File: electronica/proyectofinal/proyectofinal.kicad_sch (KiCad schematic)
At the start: 16 parts, among them J1 cnn, J2 conector alimentacion esp, J3 dht22, J4 Guva-s12s, J5 convertidor_TTL, J6 MICS-6814, K1 SRD-05VDC-SL-C, K2 SRD-05VDC-SL-C, U1 LM7833_TO220, U3 LM7805_TO220, U4 ESP32_LORA_V2.0

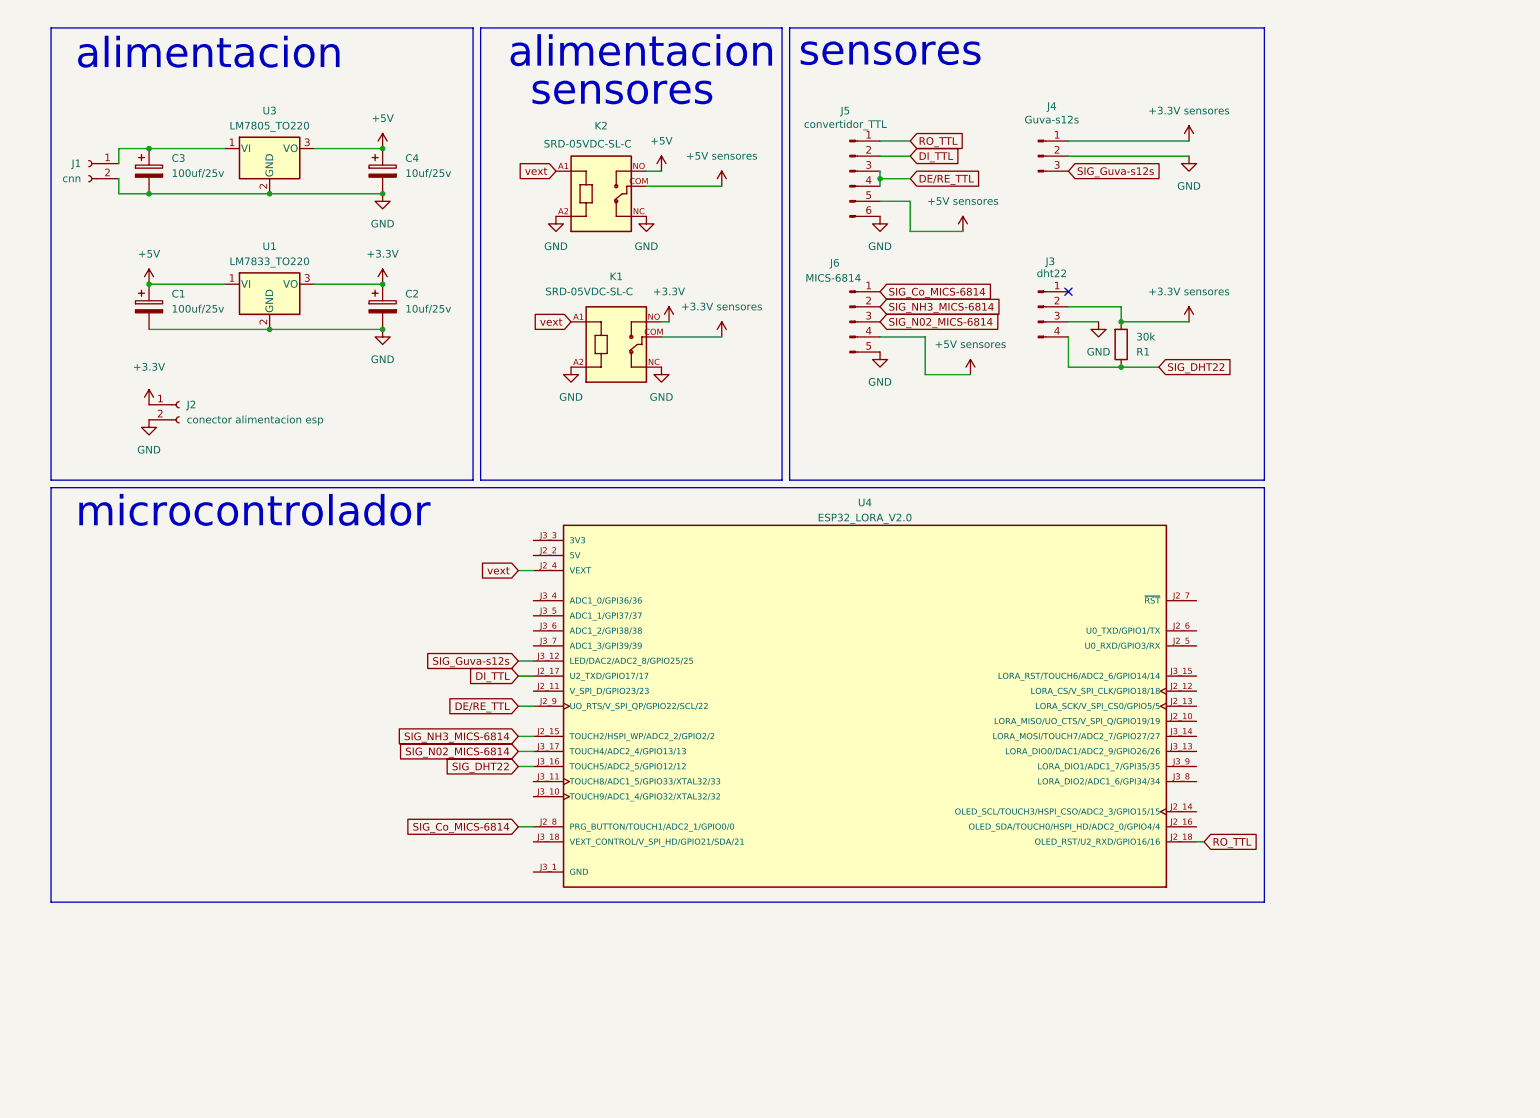
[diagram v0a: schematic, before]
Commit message: 1
1
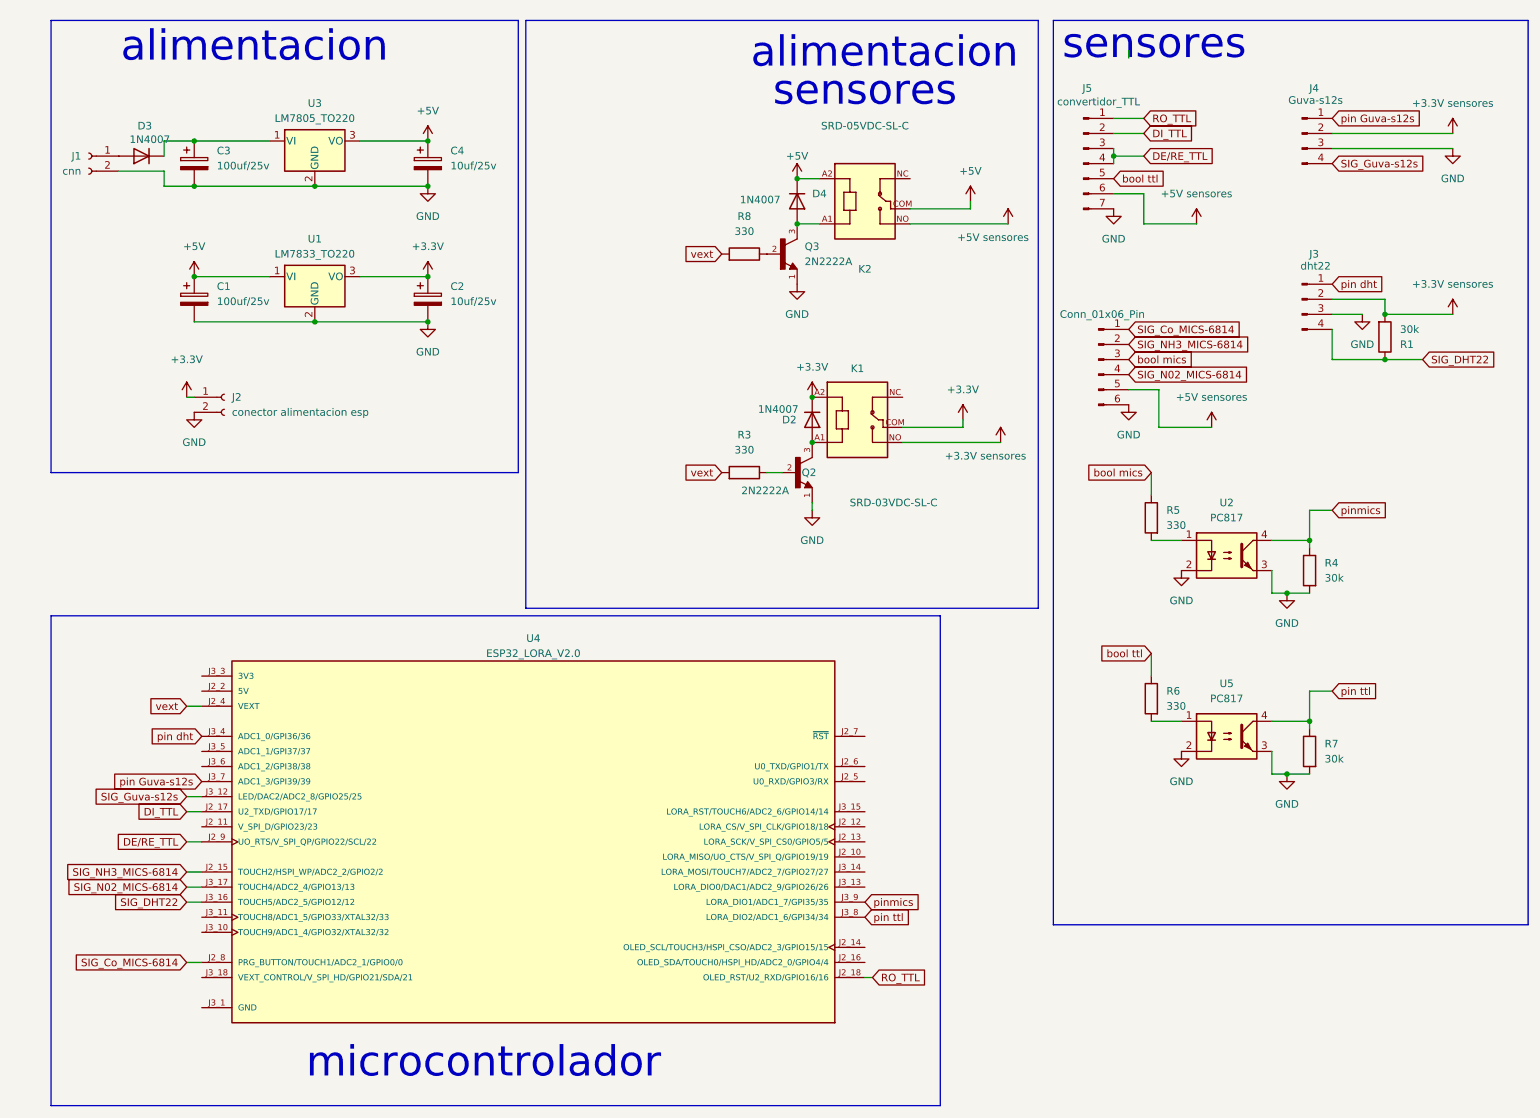
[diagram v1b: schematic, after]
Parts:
- removed J4: Guva-s12s, Connector_Molex:Molex_KK-254_AE-6410-03A_1x03_P2.54mm_Vertical, symbol Connector:Conn_01x03_Pin
- removed J5: convertidor_TTL, Connector_Molex:Molex_KK-254_AE-6410-06A_1x06_P2.54mm_Vertical, symbol Connector:Conn_01x06_Pin
- removed J6: MICS-6814, Connector_Molex:Molex_KK-254_AE-6410-05A_1x05_P2.54mm_Vertical, symbol Connector:Conn_01x05_Pin
- added D2, D3, D4: 1N4007, Diode_THT:D_DO-41_SOD81_P10.16mm_Horizontal, symbol Diode:1N4007
- added J4: Guva-s12s, Connector_Molex:Molex_KK-254_AE-6410-04A_1x04_P2.54mm_Vertical, symbol Connector:Conn_01x04_Pin
- added J5: convertidor_TTL, Connector_Molex:Molex_KK-254_AE-6410-07A_1x07_P2.54mm_Vertical, symbol Connector:Conn_01x07_Pin
- added J7: Conn_01x06_Pin, Connector_Molex:Molex_KK-254_AE-6410-06A_1x06_P2.54mm_Vertical, symbol Connector:Conn_01x06_Pin
- added Q2, Q3: 2N2222A, 2N2222A:TO92254P470H750-3, symbol 2N2222A:2N2222A
- added R3, R5, R6, R8: 330, Resistor_THT:R_Axial_DIN0207_L6.3mm_D2.5mm_P10.16mm_Horizontal, symbol Device:R
- added R4, R7: 30k, Resistor_THT:R_Axial_DIN0207_L6.3mm_D2.5mm_P10.16mm_Horizontal, symbol Device:R
- added U2, U5: PC817, Package_DIP:DIP-4_W7.62mm, symbol Isolator:PC817
- K1: value SRD-05VDC-SL-C -> SRD-03VDC-SL-C
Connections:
- net +3.3V: now also K1.A2, K1.COM, D2.1 (K); no longer K1.NO
- net +3.3V sensores: now also K1.NO, J4.2 (Pin_2); no longer K1.COM
- net +5V: now also K2.A2, K2.COM, D4.1 (K); no longer K2.NO
- net +5V sensores: now also K2.NO, J5.6 (Pin_6), J7.5 (Pin_5); no longer K2.COM
- net DE/RE_TTL: now also J5.3 (Pin_3), J5.4 (Pin_4)
- net DI_TTL: now also J5.2 (Pin_2)
- net GND: now also J4.3 (Pin_3), J5.7 (Pin_7), J7.6 (Pin_6), Q2.1, Q3.1, R4.2, R7.2, U2.2, U2.3, U5.2, U5.3; no longer K1.A2, K1.NC, K2.A2, K2.NC
- net RO_TTL: now also J5.1 (Pin_1)
- net SIG_Co_MICS-6814: now also J7.1 (Pin_1)
- net SIG_Guva-s12s: now also J4.4 (Pin_4)
- net SIG_N02_MICS-6814: now also J7.4 (Pin_4)
- net SIG_NH3_MICS-6814: now also J7.2 (Pin_2)
- net vext: now also R3.2, R8.2; no longer K1.A1, K2.A1
- net at C3.1, U3.1 (VI): now also D3.1 (K); no longer J1.1 (Pin_1)
- net pin dht: now reaches J3.1 (Pin_1)
- net pin dht: now also U4.J3_4 (ADC1_0/GPI36/36)
- net pin Guva-s12s: now reaches U4.J3_7 (ADC1_3/GPI39/39)
- net pin Guva-s12s: now also J4.1 (Pin_1)
- net pin ttl: now reaches U4.J3_8 (LORA_DIO2/ADC1_6/GPI34/34)
- net pin ttl: now also R7.1, U5.4
- net pinmics: now reaches U4.J3_9 (LORA_DIO1/ADC1_7/GPI35/35)
- net pinmics: now also R4.1, U2.4
- new net: Q2.2, R3.1
- new net: D2.2 (A), K1.A1, Q2.3
- new net: R6.2, U5.1
- new net: R5.2, U2.1
- new net: D3.2 (A), J1.1 (Pin_1)
- new net: Q3.2, R8.1
- new net: D4.2 (A), K2.A1, Q3.3
- new net bool mics: J7.3 (Pin_3), R5.1
- new net bool ttl: J5.5 (Pin_5), R6.1
- no-connect marks 1 -> 0
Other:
- moved on the sheet: C1, C2, C3, C4, J1, J2, J3, K1, R1, U1, U3, U4
